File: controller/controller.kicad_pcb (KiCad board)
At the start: 2 copper layers, 50 x 48 mm, 64 parts, among them J1 ICSP, J2 USB_B_Micro, J3 TRRS_Jack, J4 6P_ZH_connector, J5 6P_ZH_connector, SW1 RESET, U3 ATmega32U4-AU, Y1 16MHz

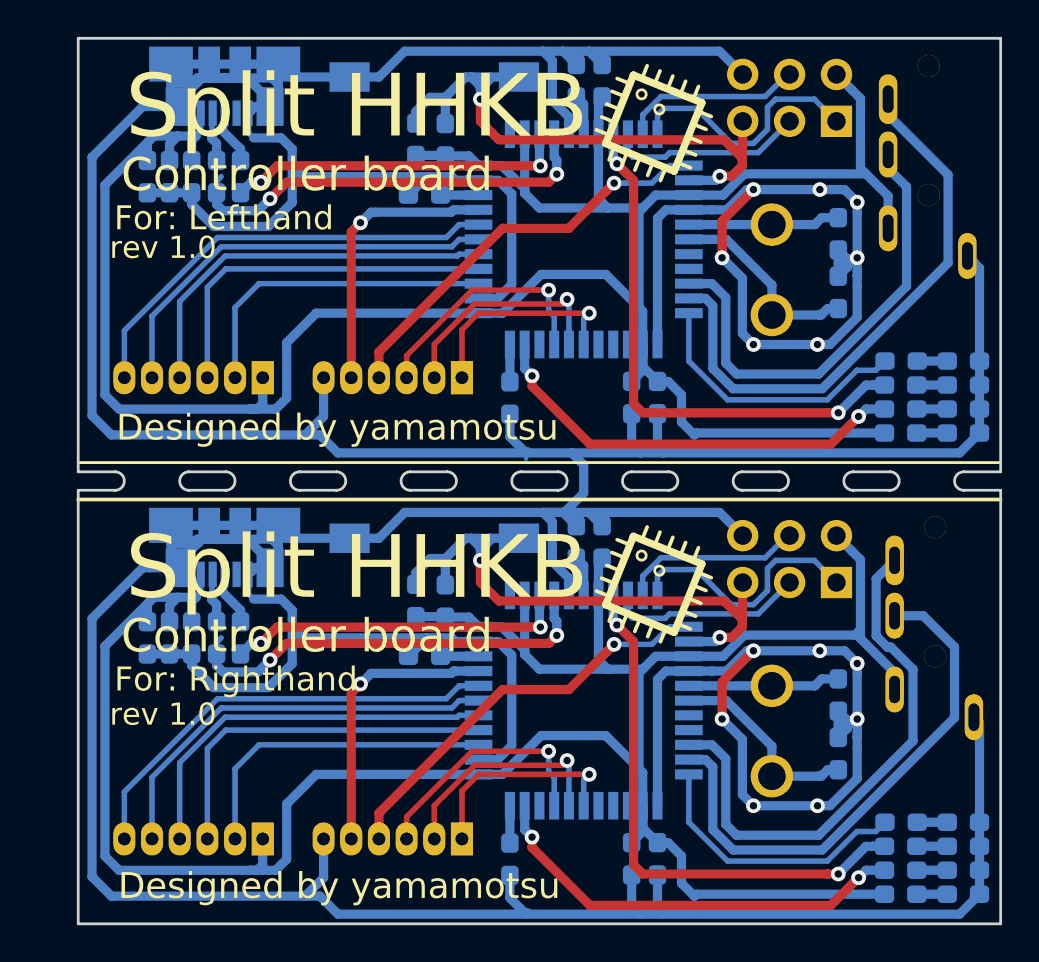
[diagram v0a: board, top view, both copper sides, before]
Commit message: [add] step files
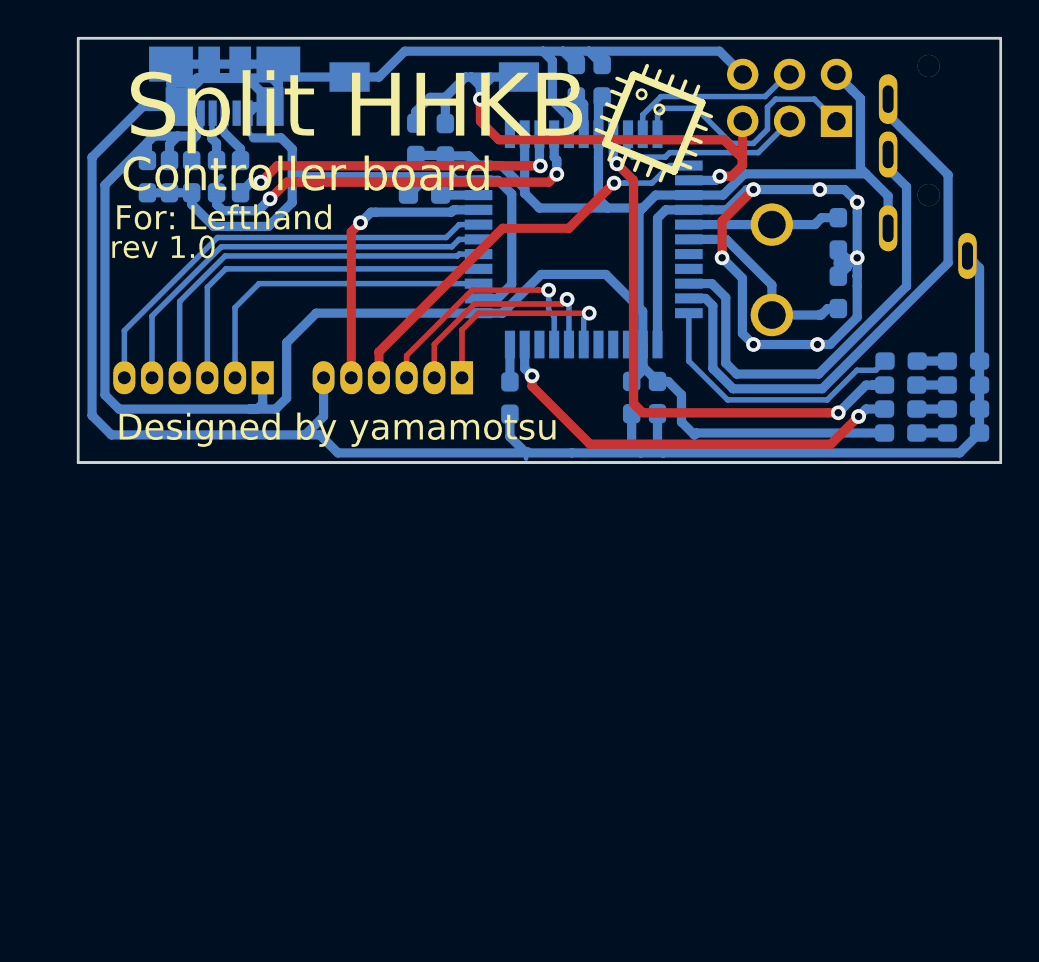
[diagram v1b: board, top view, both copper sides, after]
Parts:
- removed the C10 at (68.8, 83.5)
- removed the C11 at (78.4, 77.3)
- removed the C12 at (77.0, 77.3)
- removed the C13 at (81.4, 94.5)
- removed the C14 at (80.0, 94.5)
- removed the C15 at (55.0, 82.5)
- removed the C16 at (53.8, 82.5)
- removed the C8 at (91.2, 88.8)
- removed the C9 at (91.2, 85.6)
- removed the D1 at (69.9, 80.5)
- removed the D2 at (98.0, 95.1)
- removed the D3 at (98.0, 93.8)
- removed the D4 at (98.0, 92.5)
- removed the D5 at (98.0, 96.4)
- removed the J1 at (91.1, 79.5)
- removed the J2 at (57.9, 77.6)
- removed the J3 at (96.5, 75.0)
- removed the J4 at (60.0, 93.4)
- removed the J5 at (70.8, 93.4)
- removed the R16 at (68.3, 80.5)
- removed the R17 at (94.6, 95.1)
- removed the R18 at (94.6, 93.8)
- removed the R19 at (94.6, 92.5)
- removed the R20 at (94.6, 96.4)
- removed the R21 at (73.4, 94.5)
- removed the R22 at (58.8, 82.5)
- removed the R23 at (57.5, 82.5)
- removed the R24 at (56.1, 82.5)
- removed the REF** at (81.2, 79.6)
- removed the SW1 at (69.3, 77.1)
- removed the U3 at (77.4, 85.9)
- removed the Y1 at (87.6, 90.0)
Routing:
- net GND: track 470.8 -> 233.4 mm, vias 14 -> 7
- net +5V: track 265.1 -> 132.6 mm
- net /RESET: track 66.9 -> 33.4 mm, vias 4 -> 2
- net /Rx: track 55.0 -> 25.4 mm
- net /RXLED: track 59.0 -> 29.5 mm, vias 4 -> 2
- net /Tx: track 60.3 -> 31.1 mm
- net /DRAIN: track 48.3 -> 24.1 mm
- net /CLKLED: track 47.2 -> 23.6 mm, vias 4 -> 2
- net /D-: track 46.5 -> 23.2 mm, vias 4 -> 2
- net /MUX_EN: track 45.5 -> 22.8 mm
- net /COL_EN: track 44.8 -> 22.4 mm, vias 2 -> 1
- net /MUX_C: track 42.8 -> 21.4 mm
- net /MUX_B: track 40.0 -> 20.0 mm
- net /D+: track 37.2 -> 18.6 mm, vias 4 -> 2
- net /MUX_A: track 35.1 -> 17.5 mm
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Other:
- board size 50 x 48 mm -> 50 x 23 mm
- board text removed: "For: Righthand"
